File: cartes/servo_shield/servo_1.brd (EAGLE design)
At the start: 53 x 55.2 mm, 33 parts, among them Q1 16MHz, U1 MCP2551, U2 ADUM1400ARWZ, U3 ADUM1250ARZ, U4 ADUM1400ARWZ, X1 5V_INPUT, X2 12V_INPUT

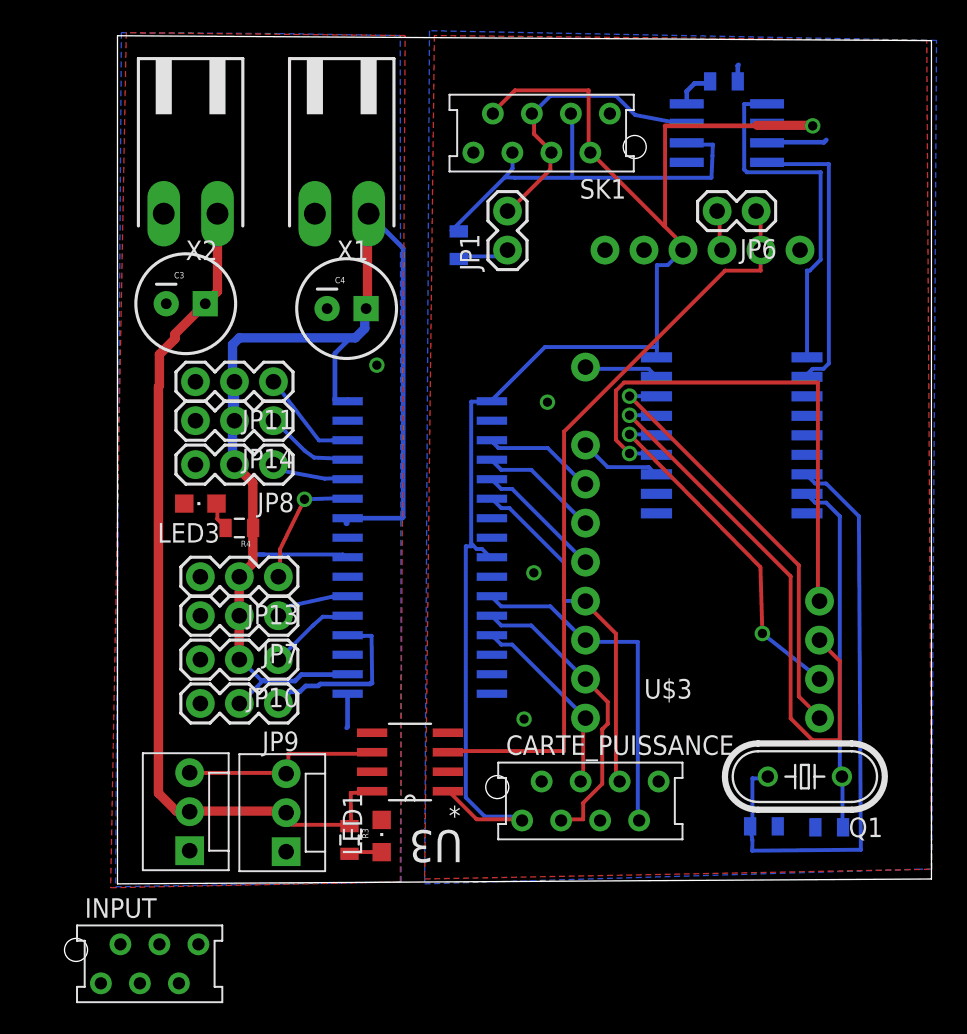
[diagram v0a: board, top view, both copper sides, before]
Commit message: ajouts carte puissance
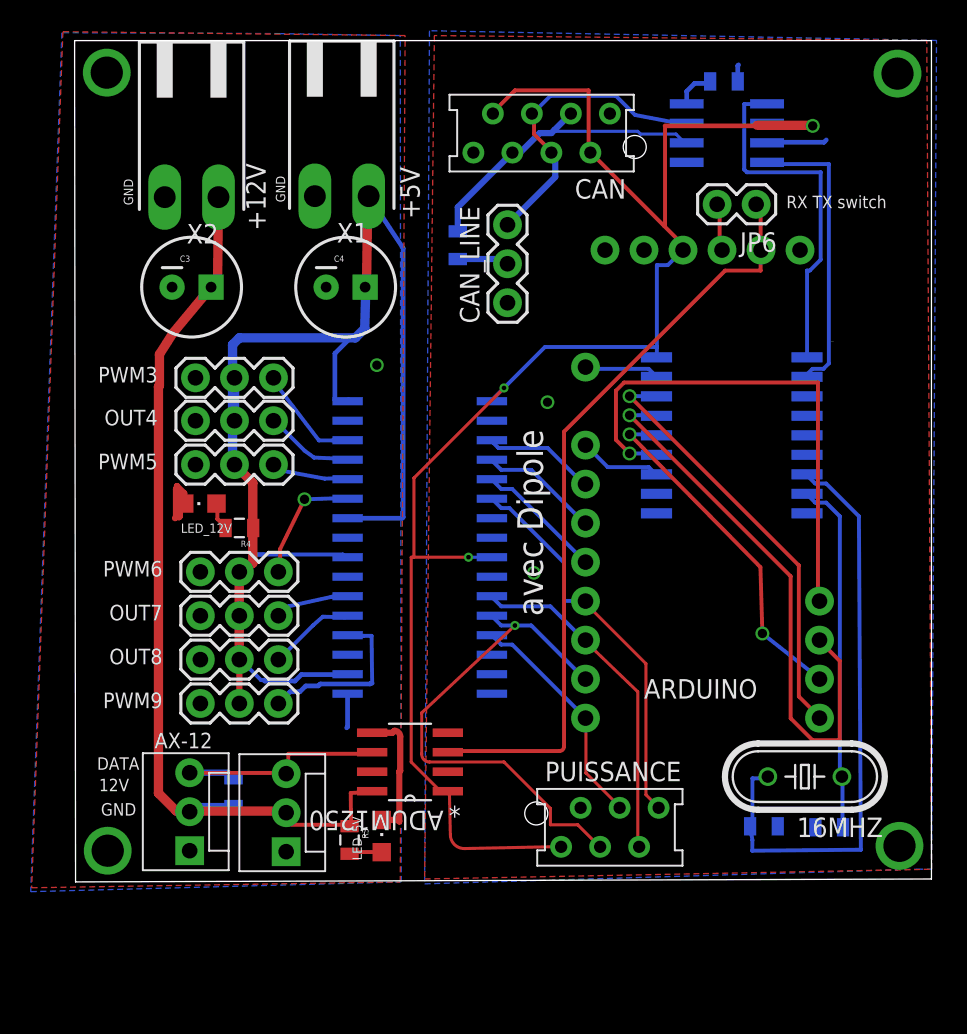
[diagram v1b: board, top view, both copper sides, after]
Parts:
- removed CARTE_PUISSANCE: (no value), jt-con-micromatch:AMP-215079-8
- removed INPUT: MMATCH-6-, jt-con-micromatch:AMP-215079-6
- removed JP1: end_lign, SparkFun-Passives:1X02
- removed JP11: PWM3, SparkFun-Connectors:1X03
- removed JP13: PWM6, SparkFun-Connectors:1X03
- added CAN_LINE: JUMPER-3PTH, SparkFun-Passives:1X03
- added PUISSANCE: MMATCH-6-, jt-con-micromatch:AMP-215079-6
- added PWM3: PWM3, SparkFun-Connectors:1X03
- added PWM6: servo_option, SparkFun-Connectors:1X03
- added R5: 10k, SparkFun-Passives:0805
- moved C4 1.40 mm to (36.4, 62.0)
- moved C3 1.14 mm to (26.4, 62.0)
- moved X1 1.14 mm to (36.2, 73.2)
- moved X2 1.08 mm to (26.4, 73.2)
- moved JP6 0.44 mm to (63.2, 67.4)
- moved R2 0.06 mm to (43.8, 64.8)
- renumbered JP10 to OUT8, JP14 to OUT4, JP7 to OUT7, JP8 to PWM5, JP9 to PWM9, LED1 to LED_5V, LED3 to LED_12V, Q1 to 16MHZ, SK1 to CAN, U$2 to CONTROLLER, U$3 to ARDUINO, U1 to TRANSCEIVER, U2 to ADUM1400_, U3 to ADUM1250, U4 to ADUM1400
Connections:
- net PWM4 renamed OUT4
- removed net C_DIR1: INPUT.3
- removed net C_DIR2: INPUT.5
- removed net C_PWM1: INPUT.4
- removed net C_PWM2: INPUT.6
- removed net PWM7: ADUM1400.3, ARDUINO.10, CARTE_PUISSANCE.7
- removed net PWM8: ADUM1400.4, ARDUINO.11, CARTE_PUISSANCE.3
- new net OUT7: ADUM1400.3, ARDUINO.10, PUISSANCE.5
- new net OUT8: ADUM1400.4, ARDUINO.11, PUISSANCE.3
- net 12V_DIRTY: now also R5.1
- net 5V_DIRTY: now also PWM3.2, PWM6.2; no longer JP11.2, JP13.2
- net CANH: now also CAN_LINE.3; no longer JP1.2
- net GND: now also PUISSANCE.2; no longer CARTE_PUISSANCE.2, INPUT.2
- net GND_DIRTY: now also PWM3.3, PWM6.3; no longer JP11.3, JP13.3
- net N$7: now also CAN_LINE.2; no longer JP1.1
- net PWM3_OUT: now also PWM3.1; no longer JP11.1
- net PWM6: now also PUISSANCE.6; no longer CARTE_PUISSANCE.6
- net PWM6_OUT: now also PWM6.1; no longer JP13.1
- net PWM9: now also PUISSANCE.4; no longer CARTE_PUISSANCE.4
- net RXTX_OUT: now also R5.2
- net VCC: now also PUISSANCE.1; no longer CARTE_PUISSANCE.1, INPUT.1
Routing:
- net OUT8: track 0.00 -> 33.6 mm, vias 0 -> 1
- net PWM7: track 22.5 -> 0.00 mm
- net OUT7: track 0.00 -> 22.2 mm
- net PWM8: track 19.7 -> 0.00 mm
- net GND_DIRTY: track 2.25 -> 18.7 mm
- net CANL: track 29.2 -> 20.4 mm
- net VCC: track 98.5 -> 105.2 mm, vias 1 -> 3
- net 12V_DIRTY: track 57.0 -> 61.4 mm
- net 5V_DIRTY: track 89.9 -> 94.2 mm
- net RXTX_OUT: track 13.2 -> 16.2 mm
- net PWM6: track 23.0 -> 25.7 mm
- net PWM9: track 12.7 -> 15.1 mm
- net CANH: track 19.2 -> 20.3 mm
- net GND: track 5.03 -> 5.22 mm, vias 3 -> 2
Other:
- board size 53 x 55.2 mm -> 55.8 x 54.8 mm
- board text added: "+12V"
- board text added: "+5V"
- board text added: "12V"
- board text added: "2014"
- board text added: "AX-12"
- board text added: "Actionneurs"
- board text added: "Carte"
- board text added: "Controller CAN"
- board text added: "DATA"
- board text added: "GND"
- board text added: "RX TX switch"
- board text added: "avec Dipole"
